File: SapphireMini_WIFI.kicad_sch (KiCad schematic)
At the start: 7 parts, among them M701 AdafruitWINC1500

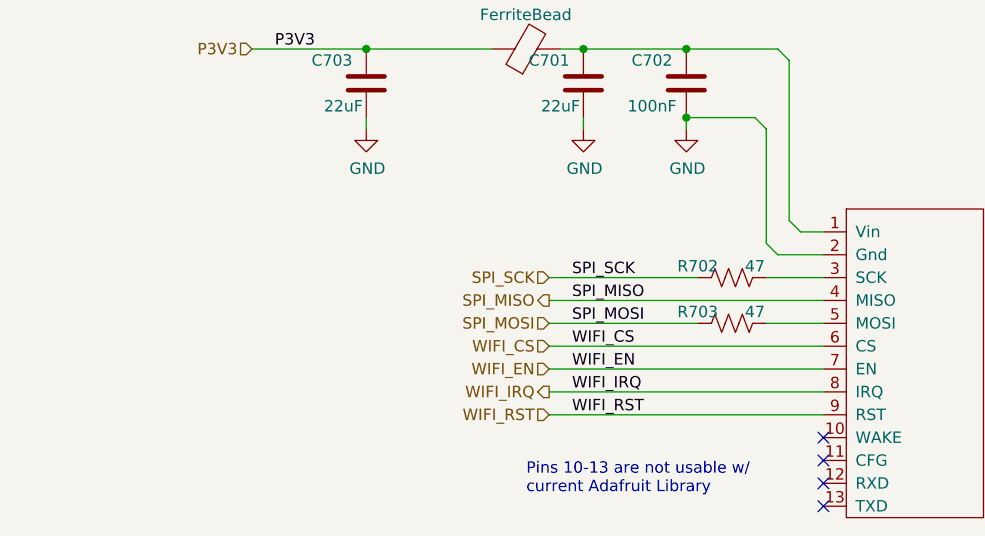
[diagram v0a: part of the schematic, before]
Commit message: Release to OSH Park
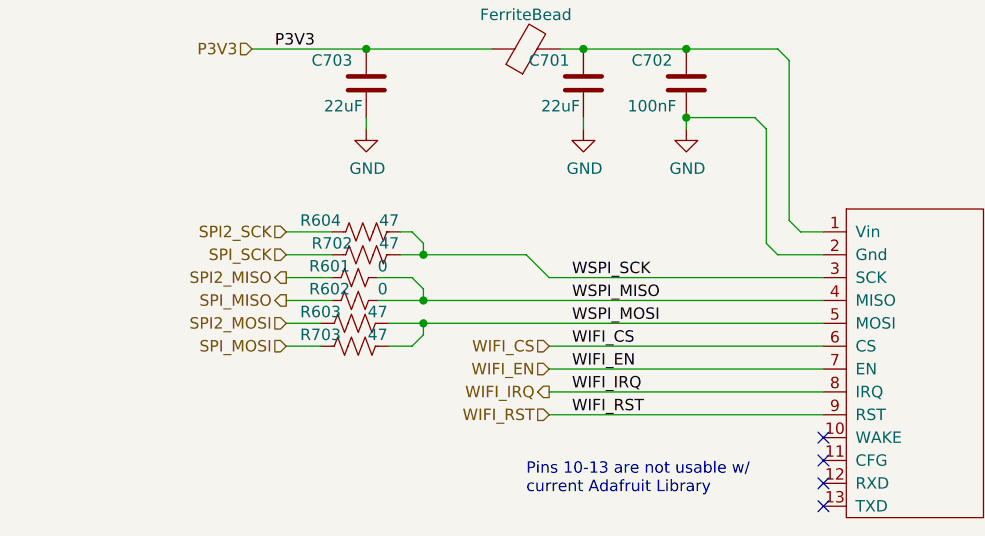
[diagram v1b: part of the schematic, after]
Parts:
- added R601, R602: 0, Resistor_SMD:R_0603_1608Metric, symbol Device:R_Small_US
- added R603, R604: 47, Resistor_SMD:R_0603_1608Metric, symbol Device:R_US
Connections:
- net SPI_MISO: now also R602.1; no longer M701.4 (MISO)
- net WSPI_SCK: now reaches M701.3 (SCK), R702.1
- net WSPI_SCK: now also R604.1
- net WSPI_MOSI: now reaches M701.5 (MOSI), R703.1
- net WSPI_MOSI: now also R603.1
- new net SPI2_MISO: R601.1
- new net SPI2_MOSI: R603.2
- new net SPI2_SCK: R604.2
- new net WSPI_MISO: M701.4 (MISO), R601.2, R602.2
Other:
- moved on the sheet: R702, R703
